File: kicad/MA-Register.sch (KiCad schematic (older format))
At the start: 6 parts, among them U57 74LS245, U58 74LS245, U59 74LS173, U60 74LS173, U61 74LS173, U62 74LS173

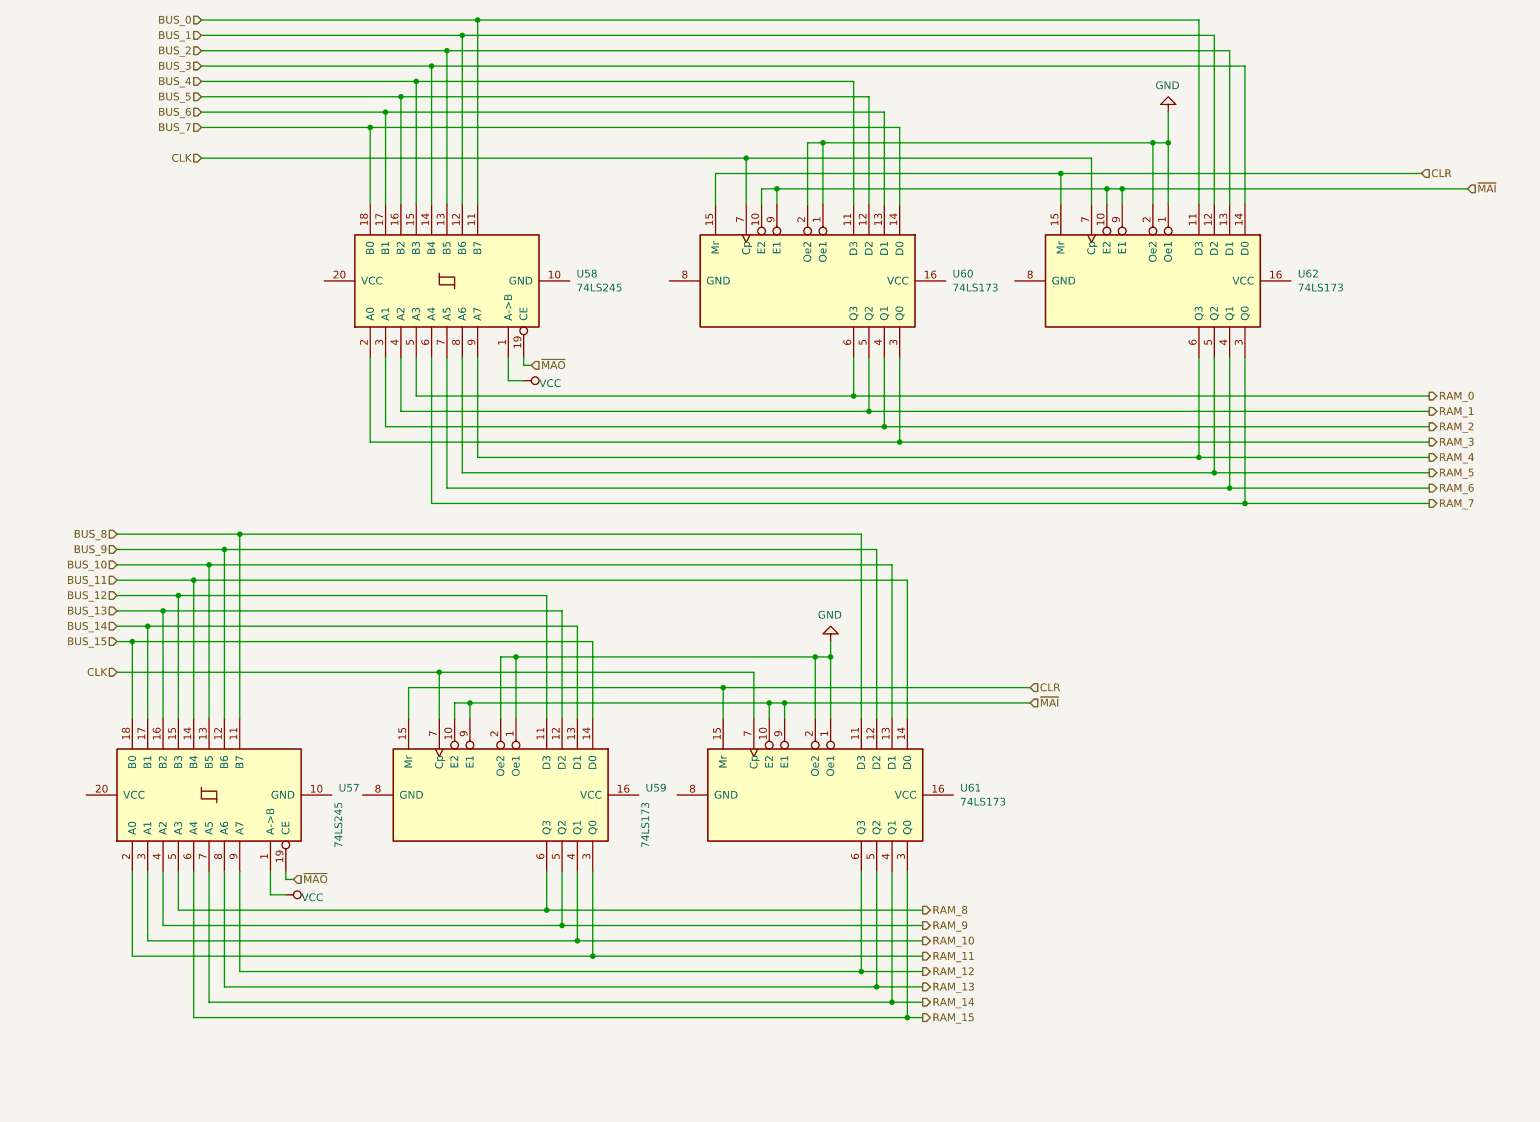
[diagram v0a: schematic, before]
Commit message: Up to v1.0 and plot
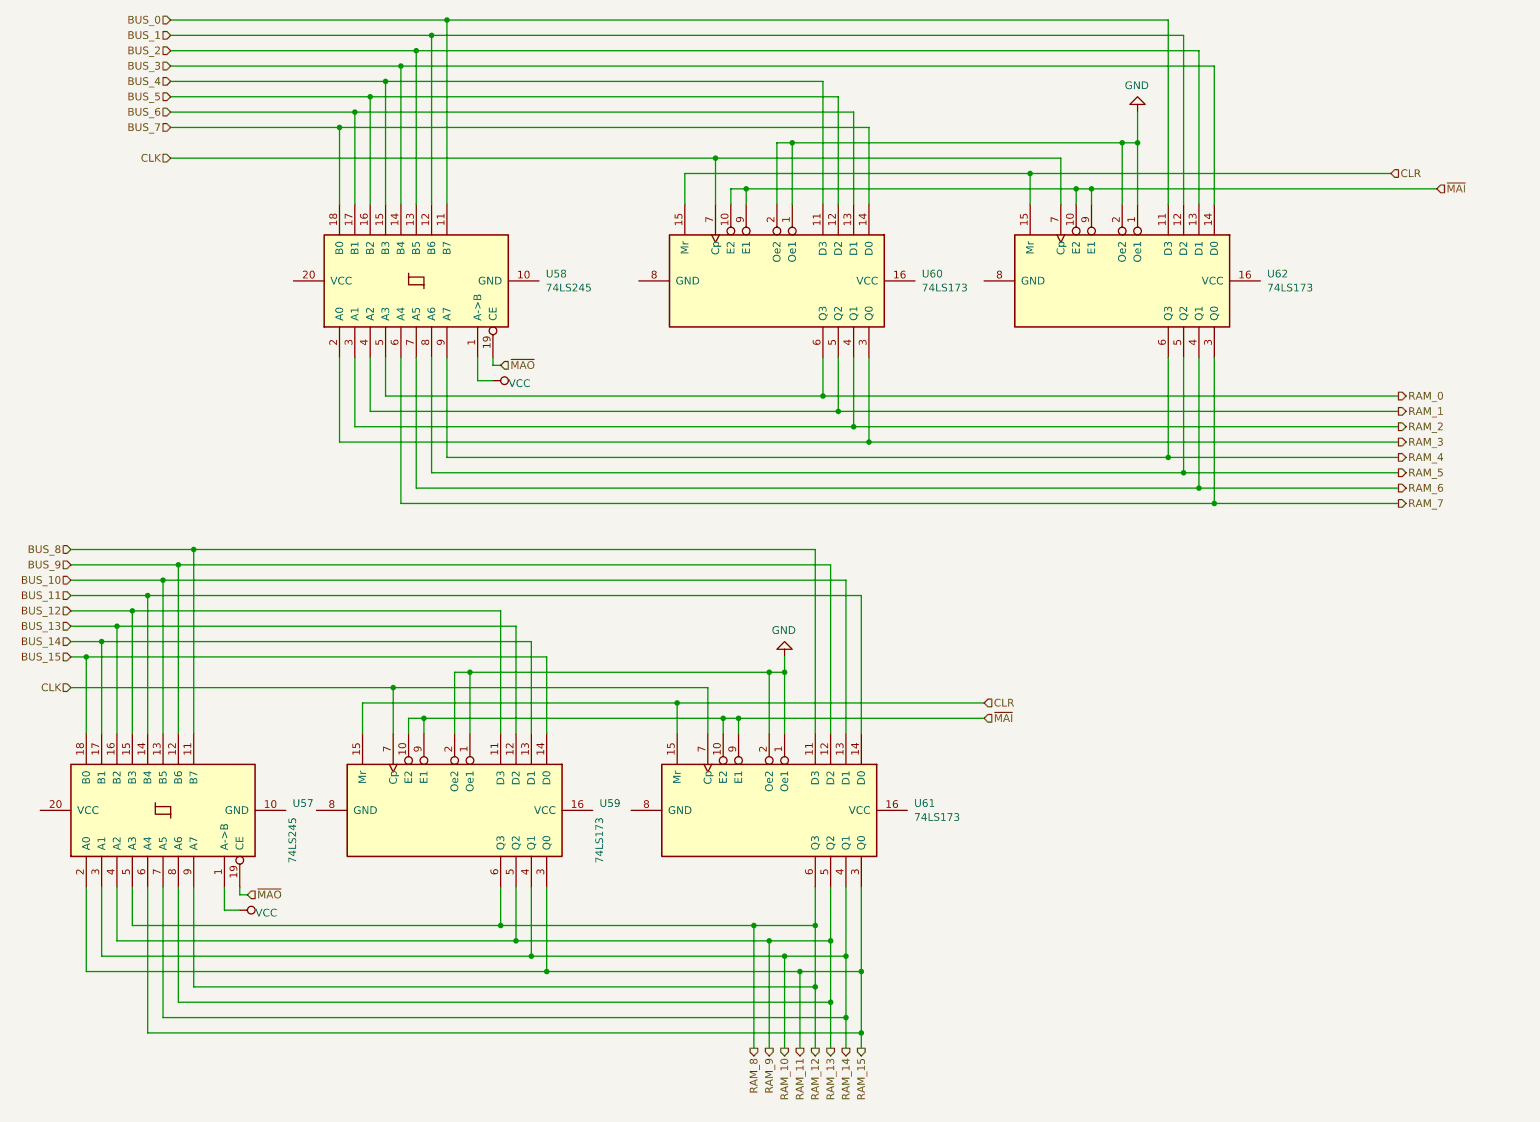
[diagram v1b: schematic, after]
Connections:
- net RAM_14 is gone; now on net RAM_10: U57.7 (A5), U61.4 (Q1)
- net RAM_15 is gone; now on net RAM_11: U57.6 (A4), U61.3 (Q0)
- net RAM_8 is gone; now on net RAM_12: U57.5 (A3), U59.6 (Q3)
- net RAM_9 is gone; now on net RAM_13: U57.4 (A2), U59.5 (Q2)
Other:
- moved on the sheet: U57, U58, U59, U60, U61, U62
